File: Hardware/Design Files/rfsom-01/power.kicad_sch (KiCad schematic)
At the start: 28 parts, among them U2 TPS51200DRCR, U3 LP8758A1E0YFFR

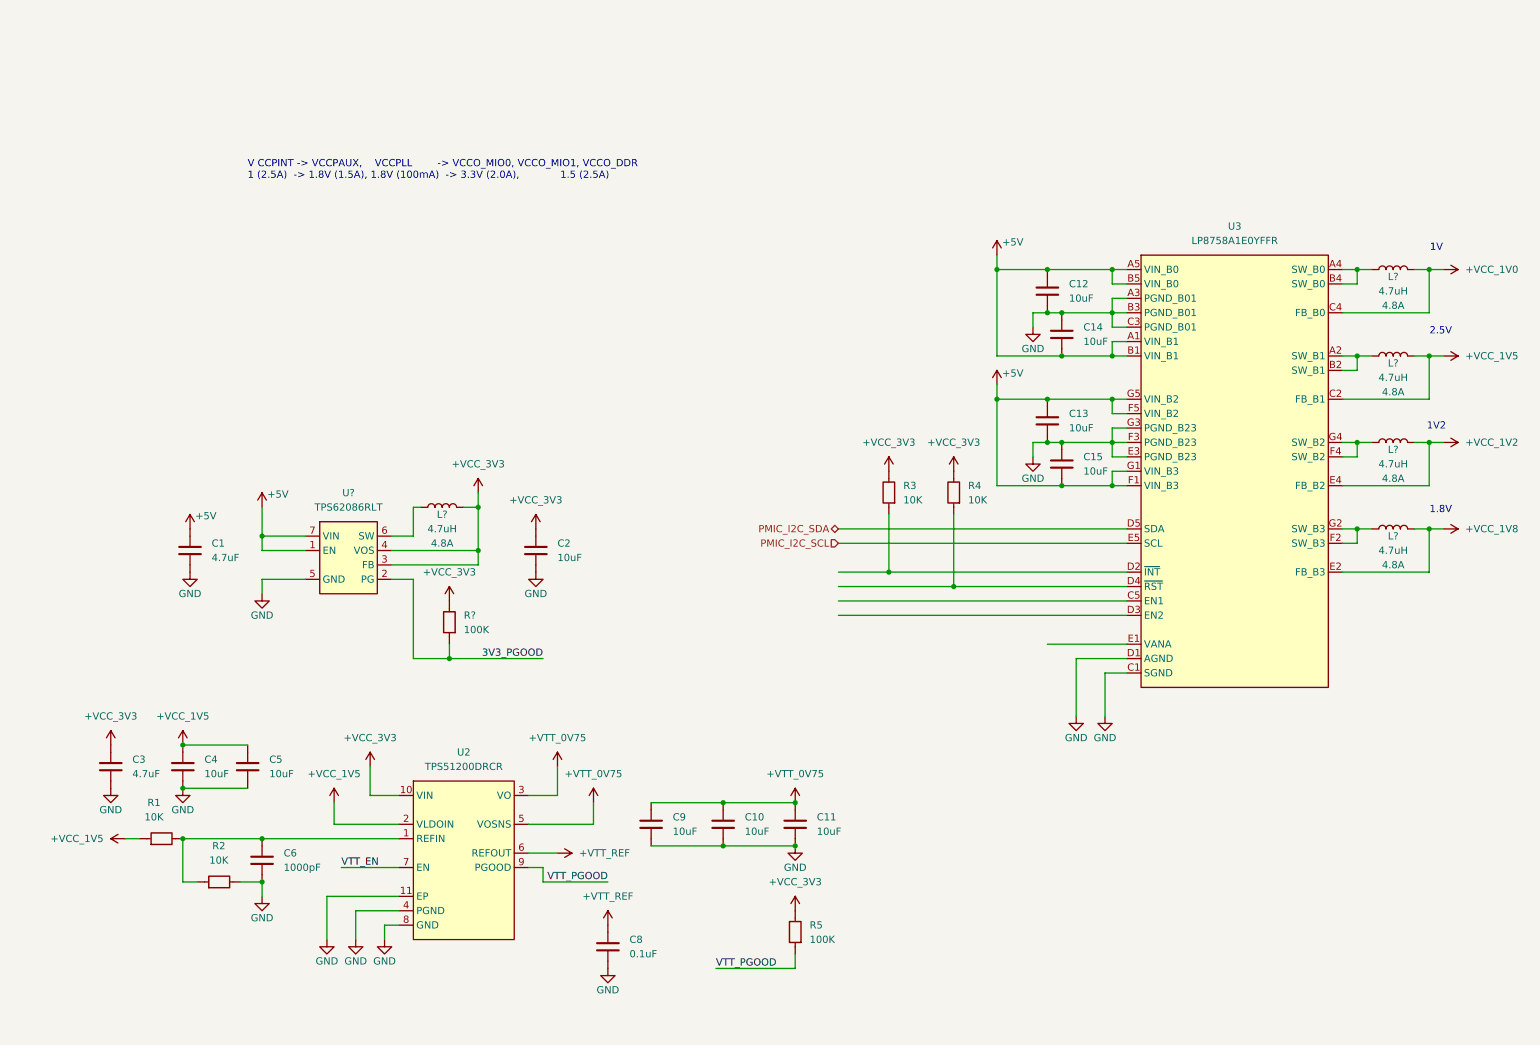
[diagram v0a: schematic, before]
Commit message: ps progress; added ftdi; mezz pinout pedinging;
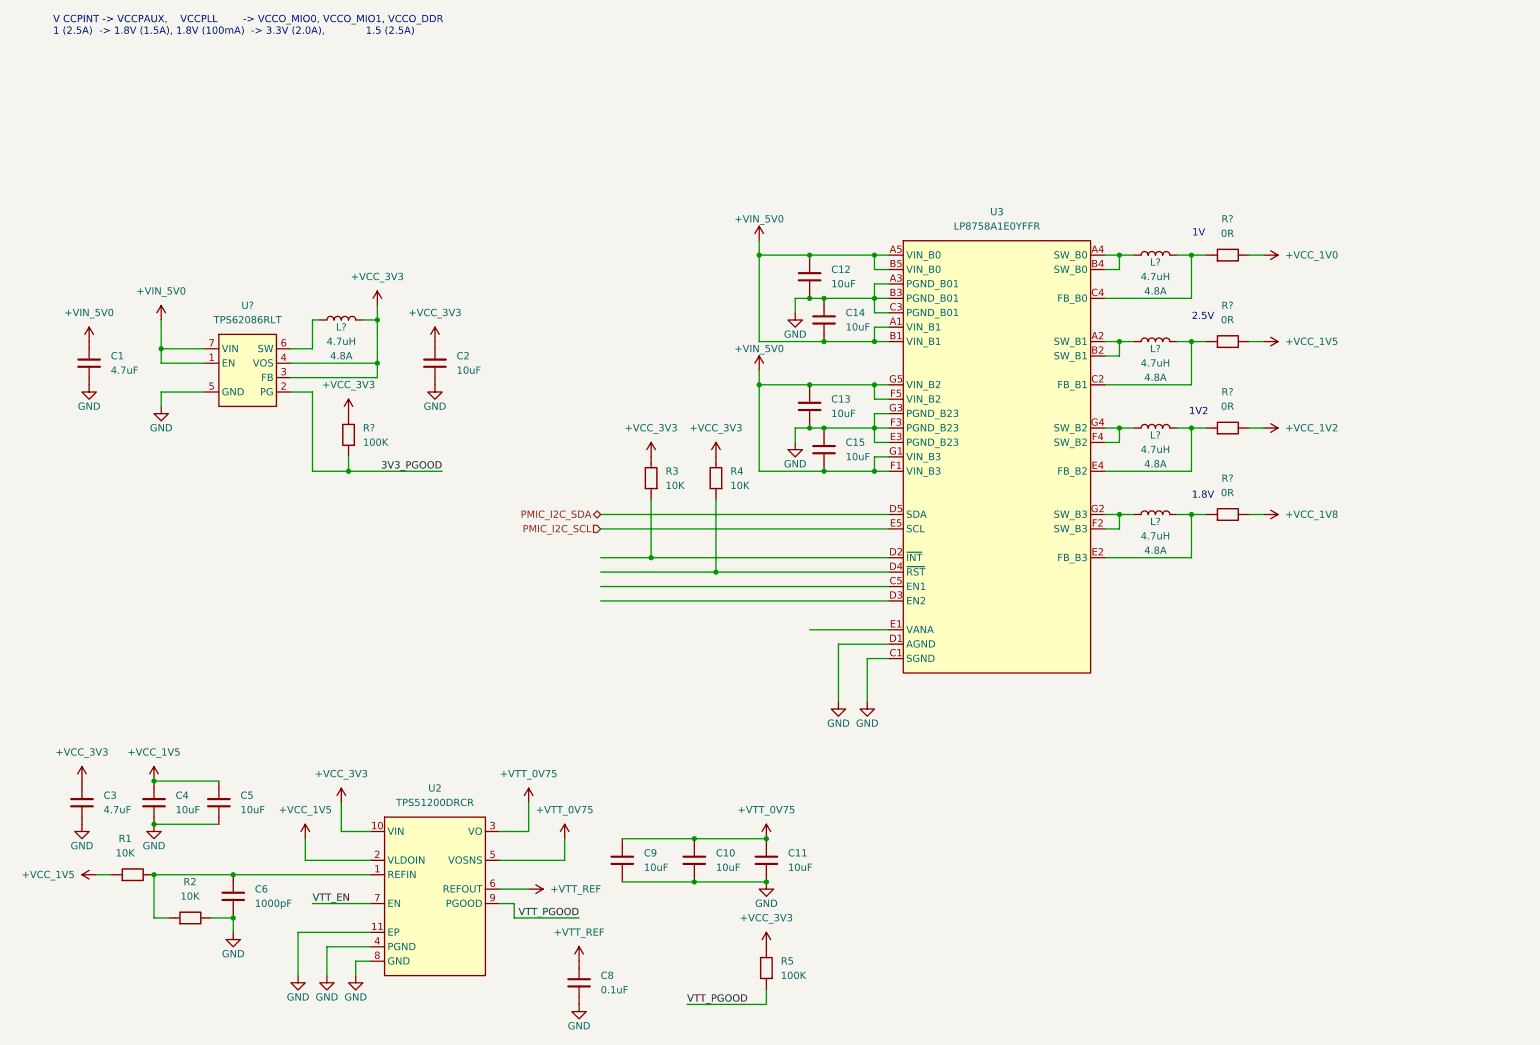
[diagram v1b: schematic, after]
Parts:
- added R? (x4): RC0603JR-070RL, Resistor_SMD:R_0603_1608Metric_Pad0.98x0.95mm_HandSolder, symbol Resistors:RC0603JR-070RL
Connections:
- net +VCC_1V0: now also R?.2; no longer L?.2, U3.C4 (FB_B0)
- net +VCC_1V2: now also R?.2; no longer L?.2, U3.E4 (FB_B2)
- net +VCC_1V5: now also R?.2; no longer L?.2, U3.C2 (FB_B1)
- net +VCC_1V8: now also R?.2; no longer L?.2, U3.E2 (FB_B3)
- net +5V renamed +VIN_5V0
- new net: L?.2, R?.1, U3.C2 (FB_B1)
- new net: L?.2, R?.1, U3.E2 (FB_B3)
- new net: L?.2, R?.1, U3.C4 (FB_B0)
- new net: L?.2, R?.1, U3.E4 (FB_B2)
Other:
- moved on the sheet: C1, C10, C11, C12, C13, C14, C15, C2, C3, C4, C5, C6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
